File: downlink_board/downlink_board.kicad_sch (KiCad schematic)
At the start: 51 parts, among them J2 SCREEN, J2 USB_C_Receptacle_USB2.0, J3 GPIO, J4 PROGRAM, SW1 MCU_{RST}, SW1 RPi_{ON}, SW2 RPi_{OFF}, U1 nRF24L01, U2 STM32F103C8Tx, U2 TPS563208DDCR, U5 AZ1117-3.3, Y1 8M

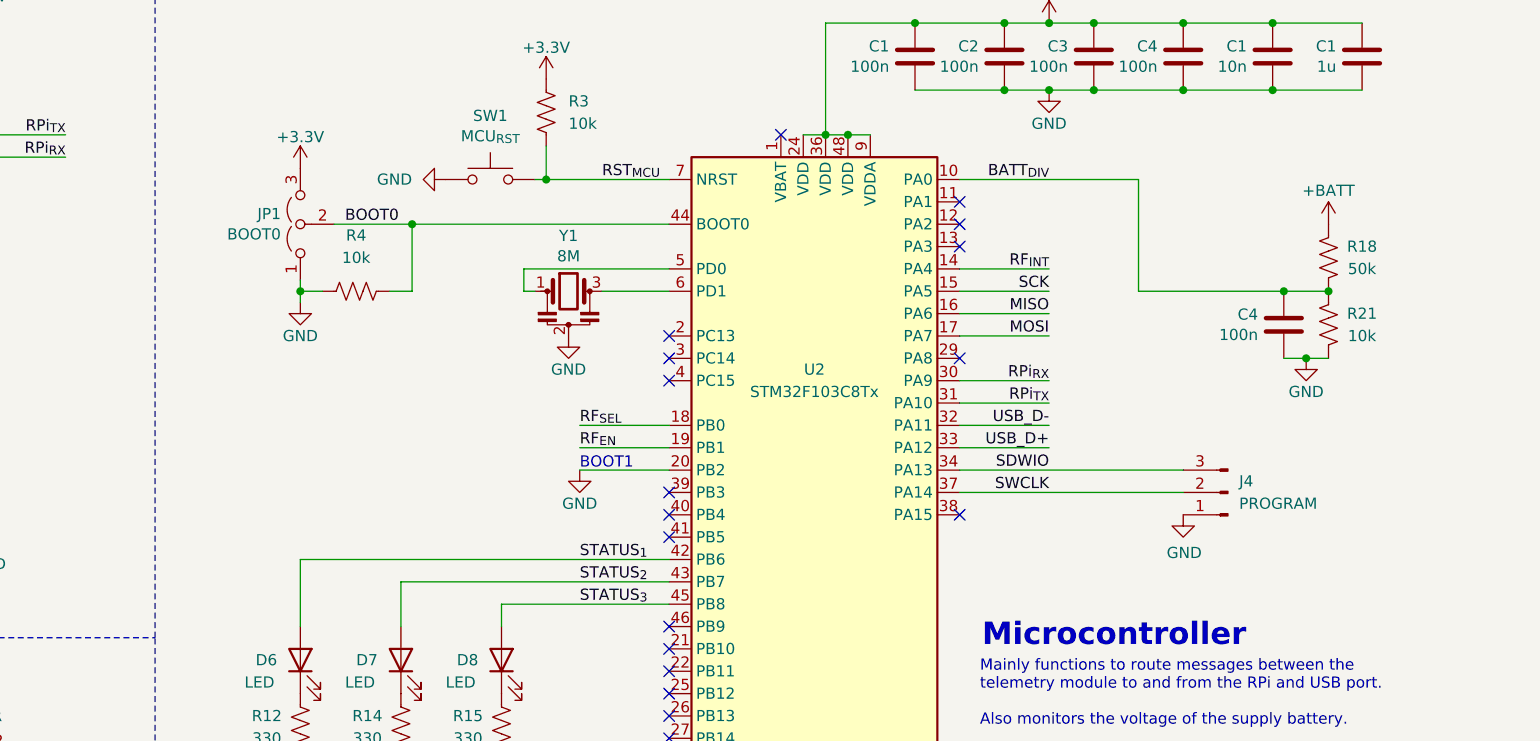
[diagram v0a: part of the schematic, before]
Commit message: Completed Rev 1.0 layout
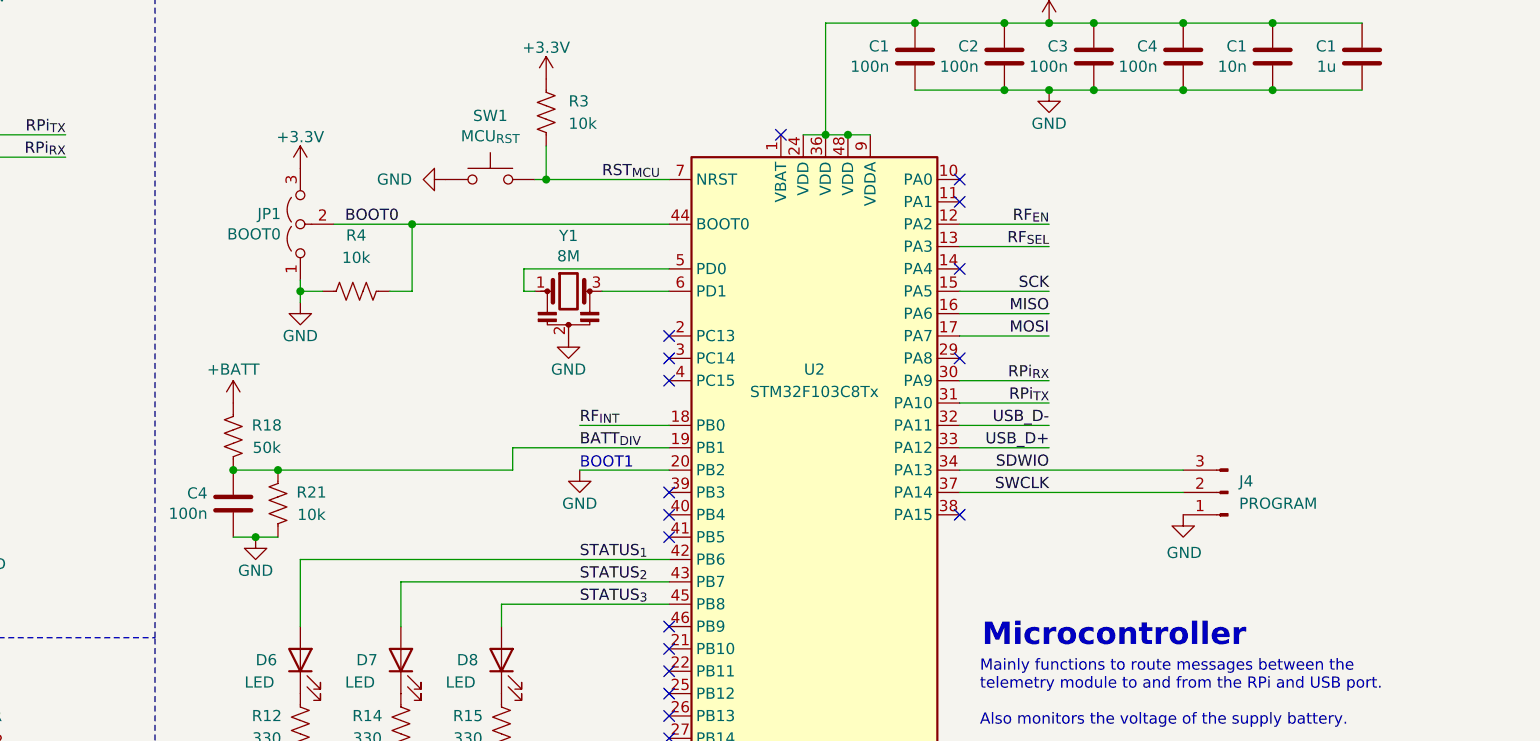
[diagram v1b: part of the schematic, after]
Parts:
- C1: footprint Capacitor_SMD:C_0805_2012Metric -> Capacitor_SMD:C_0603_1608Metric
- J4: footprint Connector_PinSocket_2.54mm:PinSocket_1x03_P2.54mm_Vertical -> Connector_PinHeader_2.54mm:PinHeader_1x03_P2.54mm_Vertical
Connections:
- net BATT_{DIV}: now also U2.19 (PB1); no longer U2.10 (PA0)
- net RF_{EN}: now also U2.12 (PA2); no longer U2.19 (PB1)
- net RF_{INT}: now also U2.18 (PB0); no longer U2.14 (PA4)
- net RF_{SEL}: now also U2.13 (PA3); no longer U2.18 (PB0)
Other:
- moved on the sheet: C4, R18, R21
